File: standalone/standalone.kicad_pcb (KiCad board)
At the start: 2 copper layers, 32 parts, among them J1 Conn_01x04_Male, J2 Conn_01x02_Male, J3 Conn_01x02_Male, J4 Conn_01x02_Male, J5 Conn_Coaxial, J6 Conn_Coaxial, J7 Conn_01x04_Male, J8 Conn_01x02_Male, J9 Conn_01x02_Male, U1 INA827AIDGK, U2 INA827AIDGK, U3 OPA2376AIDG4, U4 OPA2376AIDG4

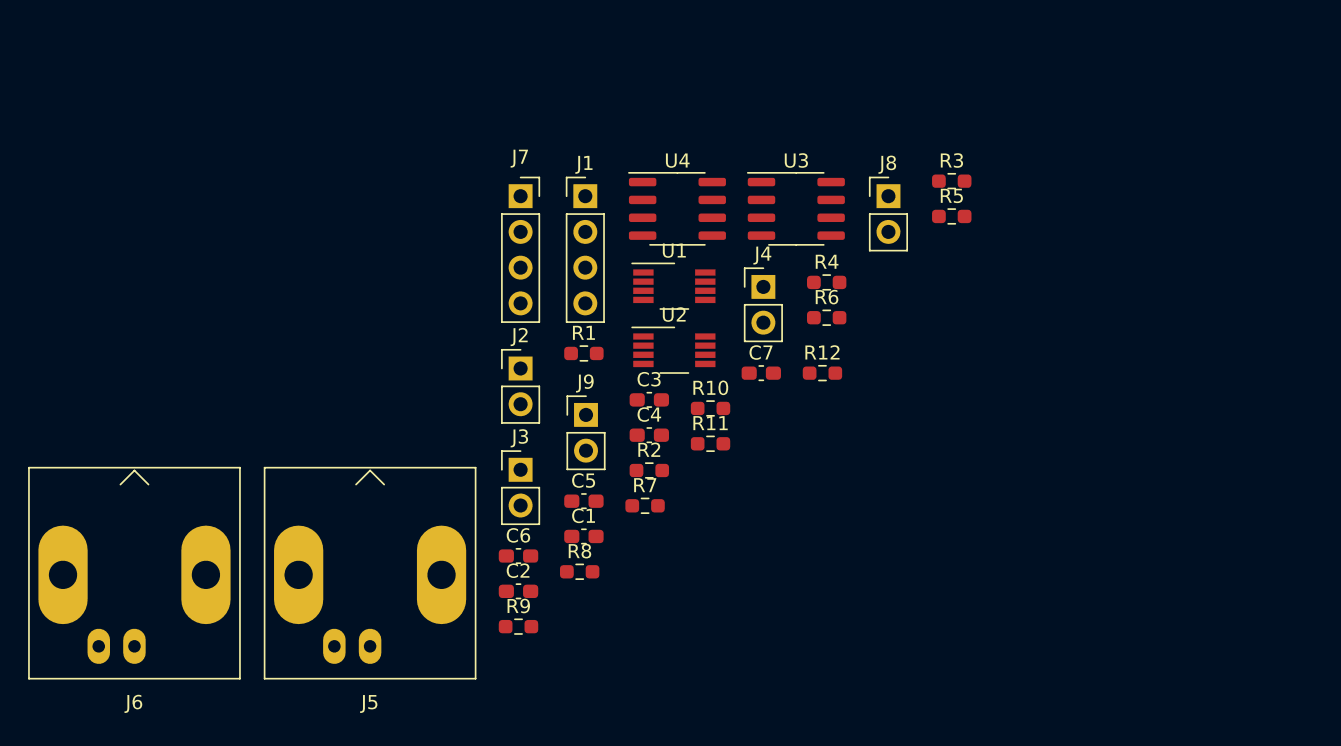
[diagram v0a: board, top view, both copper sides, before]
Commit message: layout completed
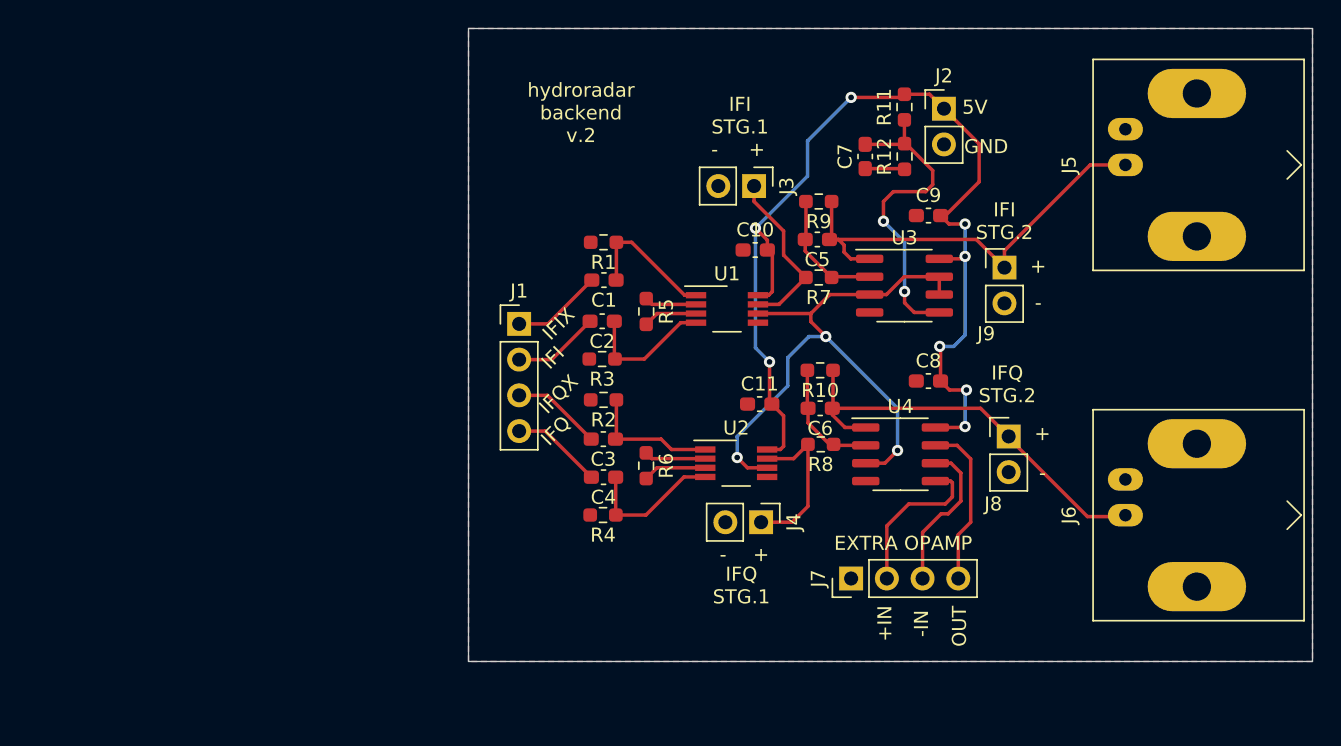
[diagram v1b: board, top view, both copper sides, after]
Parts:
- added C10: 100p, Capacitor_SMD:C_0603_1608Metric_Pad1.08x0.95mm_HandSolder, F.Cu at (120.4, 40.7)
- added C11: 100p, Capacitor_SMD:C_0603_1608Metric_Pad1.08x0.95mm_HandSolder, F.Cu at (120.7, 51.7)
- added C8: 100p, Capacitor_SMD:C_0603_1608Metric_Pad1.08x0.95mm_HandSolder, F.Cu at (132.7, 50.1)
- added C9: 100p, Capacitor_SMD:C_0603_1608Metric_Pad1.08x0.95mm_HandSolder, F.Cu at (132.7, 38.3)
- J7: footprint Connector_PinSocket_2.54mm:PinSocket_1x04_P2.54mm_Vertical -> Connector_PinHeader_2.54mm:PinHeader_1x04_P2.54mm_Vertical
- moved J6 71.1 mm to (146.7, 59.6), turned to 270 degrees
- moved J5 63.7 mm to (146.7, 34.7), turned to 270 degrees
- moved R9 37.0 mm to (124.9, 37.3), turned to 180 degrees
- moved J7 35.9 mm to (127.2, 64.1), turned to 90 degrees
- moved J2 35.3 mm to (133.8, 30.7)
- moved J9 31.5 mm to (138.1, 42.0)
- moved R3 27.9 mm to (109.5, 48.5), turned to 180 degrees
- moved R11 27.6 mm to (131.0, 30.6), turned to 90 degrees
- moved J3 26.1 mm to (120.3, 36.2), turned to 270 degrees
- moved C5 24.9 mm to (124.8, 40.0), turned to 180 degrees
- moved C6 23.9 mm to (125.0, 52.0), turned to 180 degrees
- moved U4 23.6 mm to (130.7, 55.3)
- moved R4 22.9 mm to (109.6, 59.6), turned to 180 degrees
- moved R5 22.7 mm to (112.6, 45.1), turned to 270 degrees
- moved R7 20.4 mm to (124.9, 42.7), turned to 180 degrees
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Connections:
- J1 pad 1: IFI -> IFIX
- J1 pad 2: IFIX -> IFI
- J1 pad 3: IFQ -> IFQX
- J1 pad 4: IFQX -> IFQ
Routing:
- net +5V: track 0.00 -> 76.2 mm, vias 0 -> 8
- net REF: track 0.00 -> 44.5 mm, vias 0 -> 3
- net IFI_ST2: track 0.00 -> 32.1 mm
- net IFQ_ST2: track 0.00 -> 30.1 mm
- net Net-(C7-Pad2): track 0.00 -> 23.1 mm, vias 0 -> 2
- net IFI_ST1: track 0.00 -> 12.2 mm
- net Net-(J7-Pad4): track 0.00 -> 11.8 mm
- net IFQ_ST1: track 0.00 -> 11.5 mm
- net Net-(J7-Pad2): track 0.00 -> 11.5 mm
- net Net-(J7-Pad3): track 0.00 -> 11.0 mm
- net Net-(C4-Pad1): track 0.00 -> 10.2 mm
- net Net-(C1-Pad1): track 0.00 -> 9.92 mm
- net Net-(C2-Pad1): track 0.00 -> 9.54 mm
- net Net-(C3-Pad1): track 0.00 -> 9.51 mm
- net Net-(C5-Pad2): track 0.00 -> 8.93 mm
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- added copper zone on B.Cu, net GND
- added copper zone on F.Cu, net GND
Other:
- board outline added: 60 x 45 mm
- board text added: "+"
- board text added: "+IN"
- board text added: "-"
- board text added: "-IN"
- board text added: "5V"
- board text added: "EXTRA OPAMP"
- board text added: "GND"
- board text added: "IFI"
- board text added: "IFI STG.1"
- board text added: "IFI STG.2"
- board text added: "IFIX"
- board text added: "IFQ"
- board text added: "IFQ STG.1"
- board text added: "IFQ STG.2"
- board text added: "IFQX"
- board text added: "OUT"
- board text added: "https://github.com/giocic2/BGT24MTR11-backend"
- board text added: "hydroradar backend v.2"
